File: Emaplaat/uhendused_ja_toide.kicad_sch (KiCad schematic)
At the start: 25 parts, among them IC4 FT232RNL-TUBE, IC5 TPS54429PWPR, J5 USB4216-03-A, J6 USB-A-S-VT, J7 USB-A-S-VT, J8 Barrel_Jack

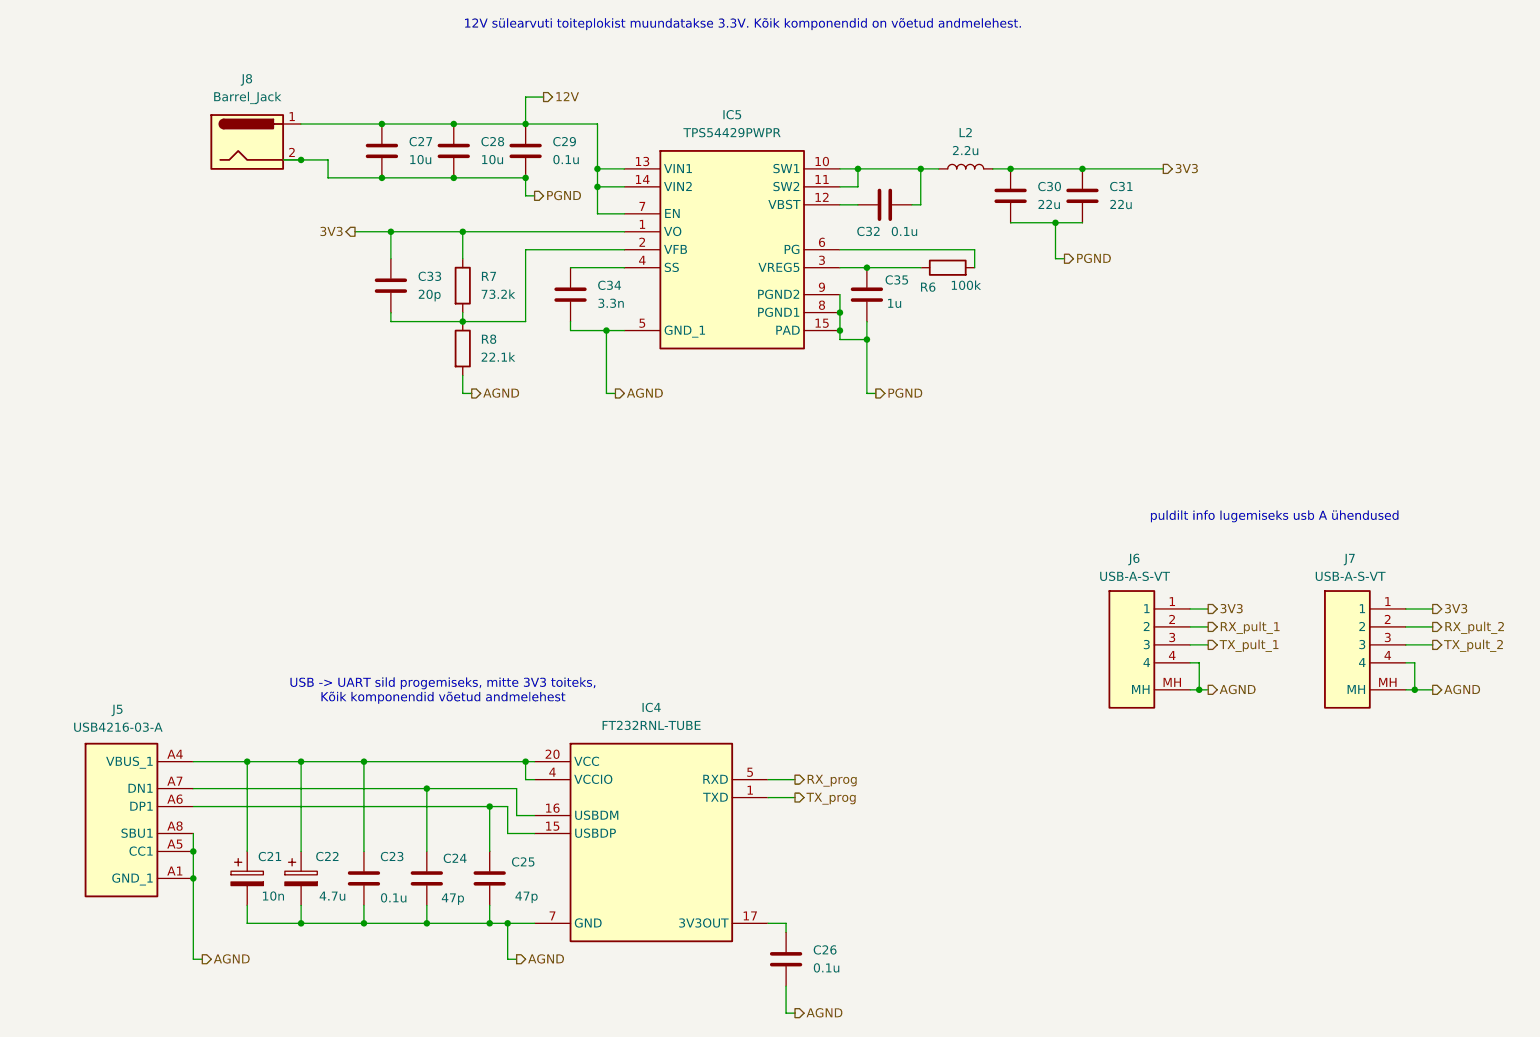
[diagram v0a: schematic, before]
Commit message: cleanoupp T__W
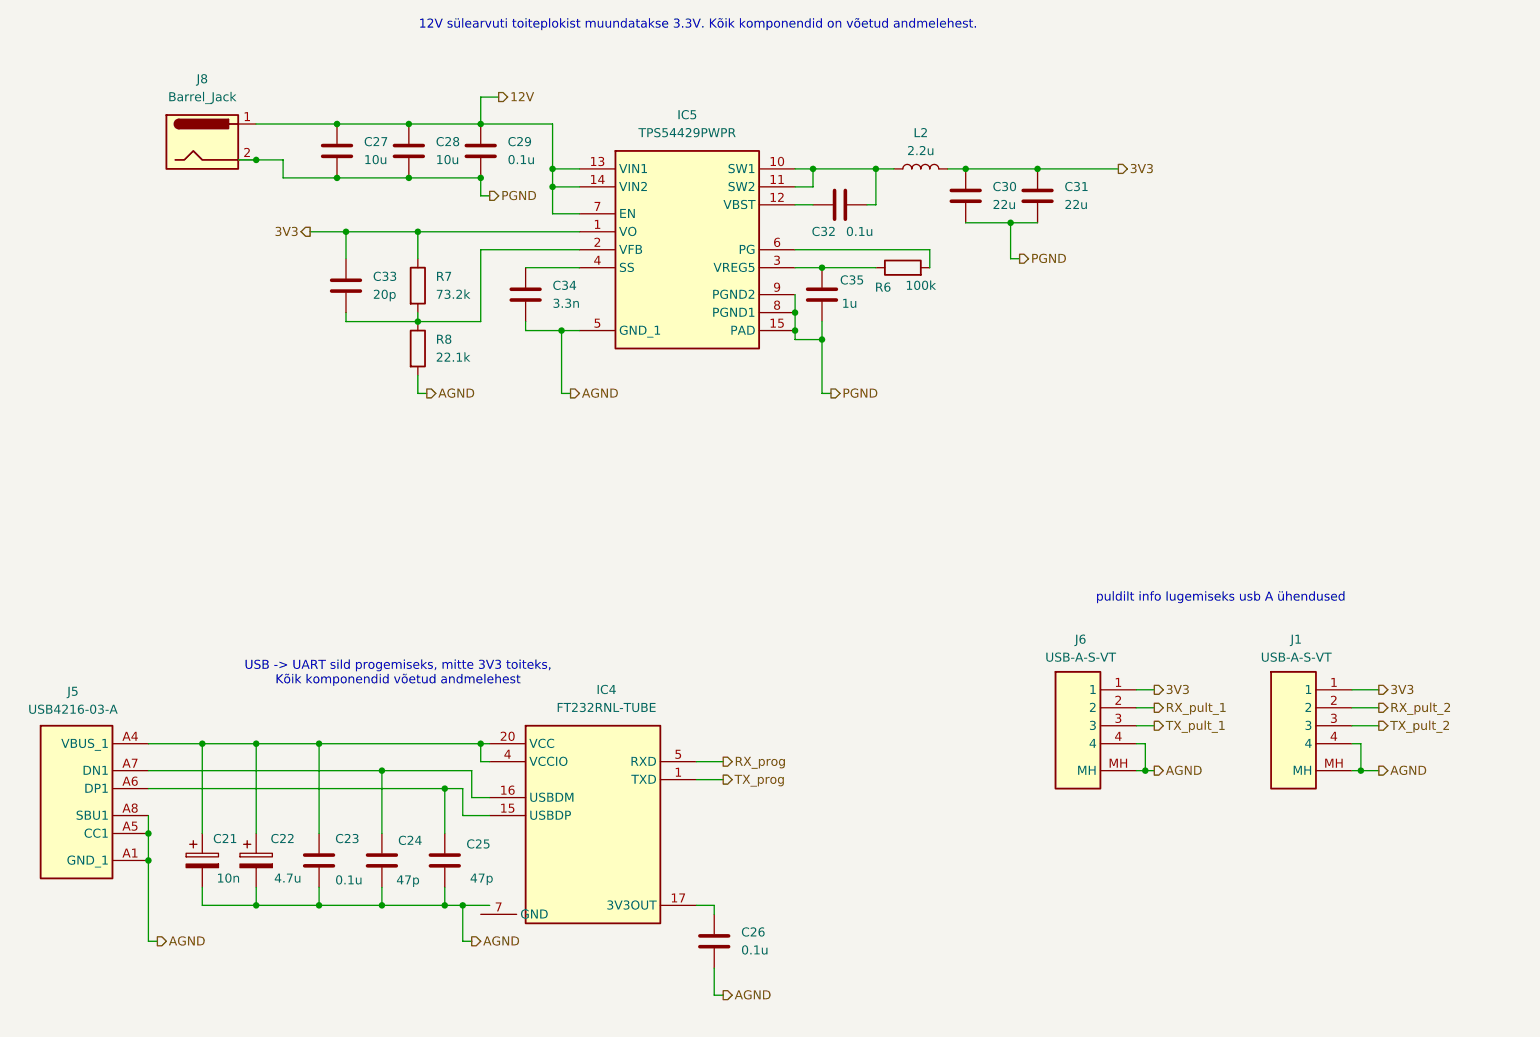
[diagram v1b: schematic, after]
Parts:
- removed J7: USB-A-S-VT, USBASVT, symbol USB-A-S-VT:USB-A-S-VT
- added J1: USB-A-S-VT, USBASVT, symbol USB-A-S-VT:USB-A-S-VT
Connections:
- net 3V3: now also J1.1
- net AGND: now also J1.4, J1.MH, J1.MH1
- net RX_pult_2: now also J1.2
- net TX_pult_2: now also J1.3
- net at IC4.19 (RESET#): now also IC4.24 (NC_2), IC4.27 (OSCI), IC4.8 (NC_1)
- net TEST: now reaches IC4.26 (TEST)
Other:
- moved on the sheet: C21, C22, C23, C24, C25, C26, C27, C28, C29, C30, C31, C32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
